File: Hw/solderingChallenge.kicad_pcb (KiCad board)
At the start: 2 copper layers, 33.5 x 33.5 mm, 28 parts, among them J1 ISP, U1 ATtiny85-20SU

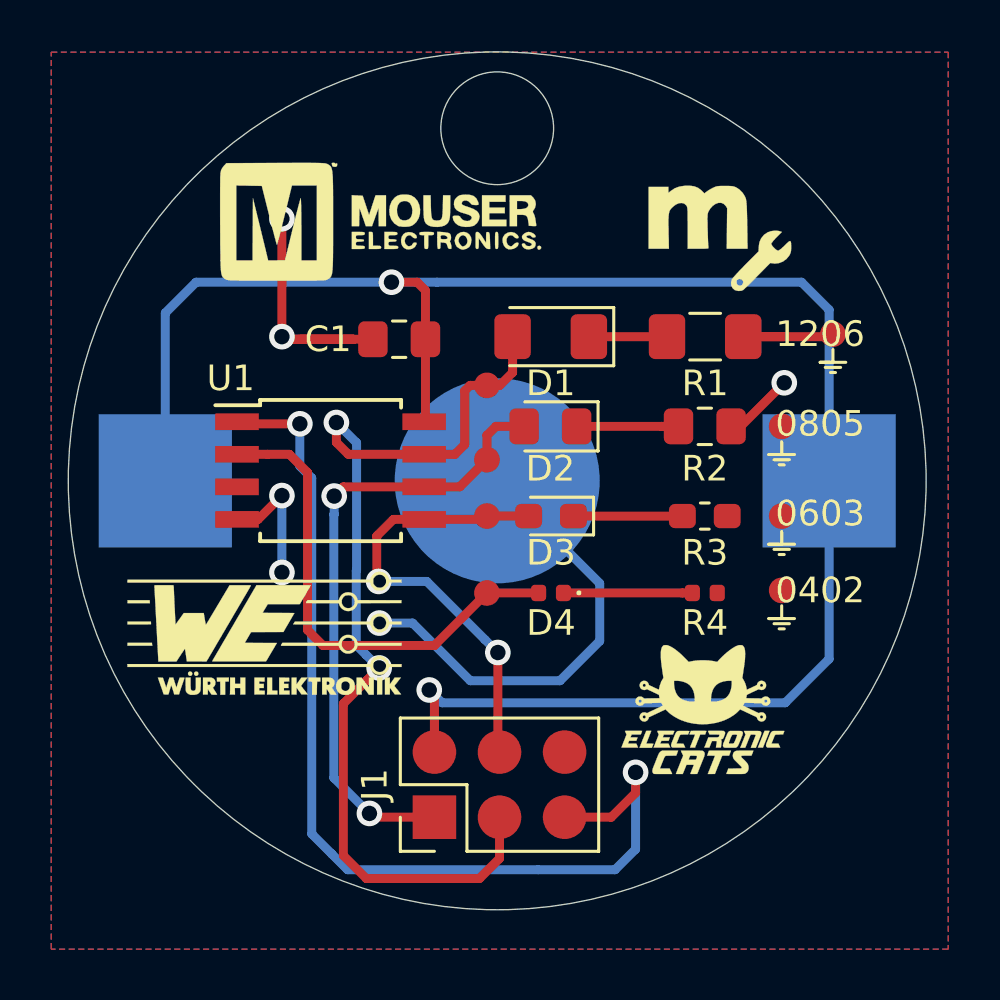
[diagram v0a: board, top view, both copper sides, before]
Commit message: feat(Hw):Added_Puya_PCB
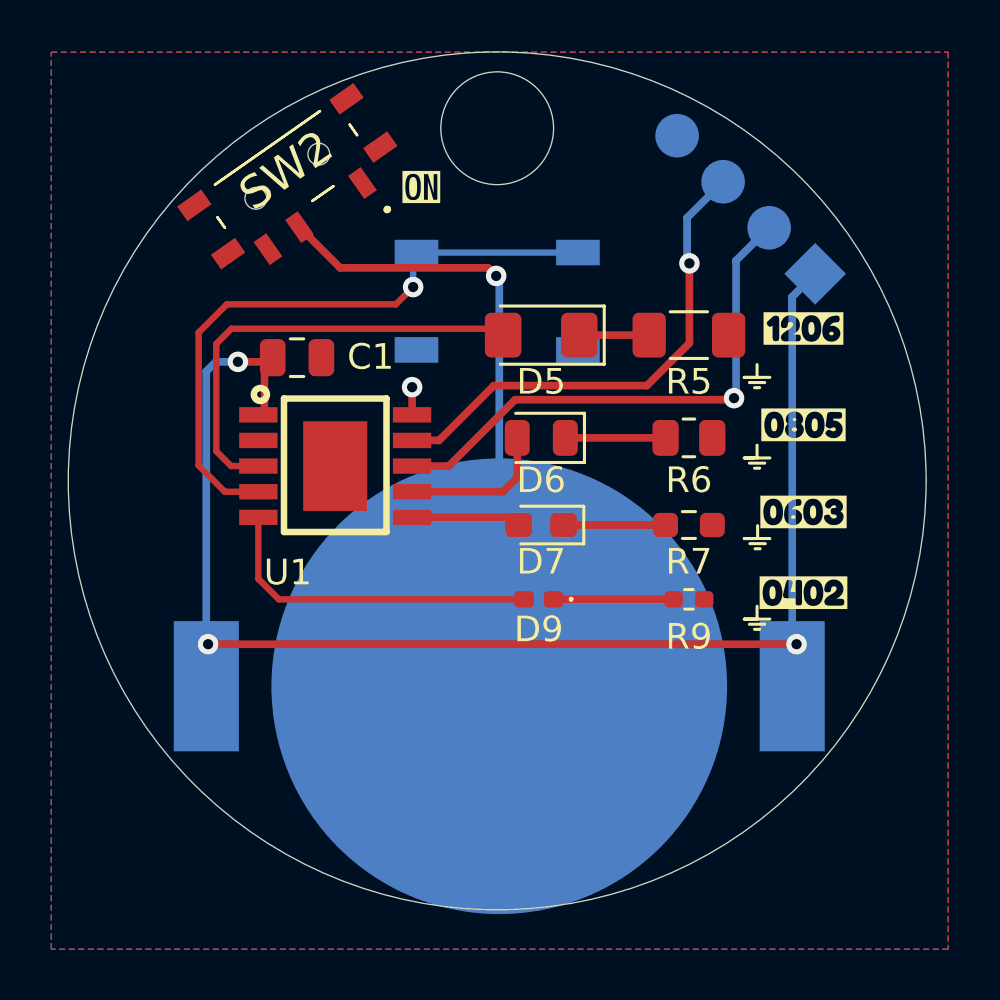
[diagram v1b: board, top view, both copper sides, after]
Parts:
- removed D1: 1206, LED_SMD:LED_1206_3216Metric_Pad1.42x1.75mm_HandSolder
- removed D2: 0805, LED_SMD:LED_0805_2012Metric_Pad1.15x1.40mm_HandSolder
- removed D3: 0603, LED_SMD:LED_0603_1608Metric_Pad1.05x0.95mm_HandSolder
- removed D4: 0402, LED_SMD:LED_0402_1005Metric
- removed the G*** at (133.6, 88.9)
- removed the G*** at (133.3, 85.2)
- removed the G*** at (150.4, 88.2)
- removed the G*** at (130.4, 73.0)
- removed the G*** at (151.4, 89.1)
- removed the G*** at (137.8, 69.1)
- removed the G*** at (142.6, 92.3)
- removed the G*** at (150.2, 69.0)
- removed J1: ISP, Connector_PinHeader_2.54mm:PinHeader_2x03_P2.54mm_Vertical
- removed R1: 1206, Resistor_SMD:R_1206_3216Metric_Pad1.42x1.75mm_HandSolder
- removed R2: 0805, Resistor_SMD:R_0805_2012Metric_Pad1.15x1.40mm_HandSolder
- removed R3: 0603, Resistor_SMD:R_0603_1608Metric_Pad1.05x0.95mm_HandSolder
- removed R4: 0402, Resistor_SMD:R_0402_1005Metric
- removed TP1: PB0, TestPoint:TestPoint_Pad_1.0x1.0mm
- removed TP10, TP6, TP7, TP8: GND, Connectors_EC:TestPoint_Pad_1.0x1.0mm
- removed TP2: PB1, Connectors_EC:TestPoint_Pad_1.0x1.0mm
- removed TP3: PB2, Connectors_EC:TestPoint_Pad_1.0x1.0mm
- removed TP4: PB3, Connectors_EC:TestPoint_Pad_1.0x1.0mm
- added D5: Green, LED_SMD:LED_1206_3216Metric_Pad1.42x1.75mm_HandSolder, F.Cu at (144.1, 73.5)
- added D6: Red, LED_SMD:LED_0805_2012Metric, F.Cu at (144.1, 77.5)
- added D7: Blue, LED_SMD:LED_0603_1608Metric_Pad1.05x0.95mm_HandSolder, F.Cu at (144.1, 81.0)
- added D9: Yellow, LED_SMD:LED_0402_1005Metric_Pad0.77x0.64mm_HandSolder, F.Cu at (144.0, 83.8)
- added G***: LOGO, Aesthetics:pcbway_13x4, F.Cu at (142.4, 88.5)
- added G***: LOGO, Aesthetics:electronic_cats_logo_4x3, F.Cu at (142.5, 92.6)
- added J2: SWD, Connector_PinHeader_2.54mm:PinHeader_1x04_P2.54mm_Vertical, B.Cu at (154.8, 71.1)
- added R5: 330R, Resistor_SMD:R_1206_3216Metric_Pad1.30x1.75mm_HandSolder, F.Cu at (149.9, 73.5)
- added R6: 330R, Resistor_SMD:R_0805_2012Metric, F.Cu at (149.9, 77.5)
- added R7: 330R, Resistor_SMD:R_0603_1608Metric_Pad0.98x0.95mm_HandSolder, F.Cu at (149.9, 81.0)
- added R9: 330R, Resistor_SMD:R_0402_1005Metric_Pad0.72x0.64mm_HandSolder, F.Cu at (149.9, 83.8)
- added SW1: SW_RST, Button_Switch_SMD:SW_SPST_TL3342, B.Cu at (142.4, 72.2)
- added SW2: On, solderingChallenge:MSK12C02, F.Cu at (134.2, 67.3)
- added kibuzzard-67914DBF: G***, kibuzzard-67914DBF, F.Cu at (154.3, 73.3)
- added kibuzzard-67914DD8: G***, kibuzzard-67914DD8, F.Cu at (154.3, 77.0)
- added kibuzzard-67914DE9: G***, kibuzzard-67914DE9, F.Cu at (154.3, 80.4)
- added kibuzzard-67914E01: G***, kibuzzard-67914E01, F.Cu at (154.3, 83.6)
- added kibuzzard-67916211: G***, kibuzzard-67916211, F.Cu at (129.1, 79.0)
- added kibuzzard-6791629E: G***, kibuzzard-6791629E, F.Cu at (129.1, 79.0)
- added kibuzzard-67916383: G***, kibuzzard-67916383, B.Cu at (153.0, 73.0)
- added kibuzzard-679163A9: G***, kibuzzard-679163A9, B.Cu at (149.4, 69.4)
- added kibuzzard-679163CD: G***, kibuzzard-679163CD, B.Cu at (151.2, 71.2)
- added kibuzzard-679168C7: G***, kibuzzard-679168C7, B.Cu at (156.0, 78.8)
- added kibuzzard-679168F3: G***, kibuzzard-679168F3, B.Cu at (147.6, 67.5)
- added kibuzzard-67916B62: G***, kibuzzard-67916B62, F.Cu at (139.4, 67.8)
- BT1: footprint Connectors_EC:79523141 -> solderingChallenge:BAT-HLD-001
- C1: footprint Capacitor_SMD:C_0805_2012Metric_Pad1.15x1.40mm_HandSolder -> Capacitor_SMD:C_0805_2012Metric
- U1: value ATtiny85-20SU -> PY32F002AA15M6TU; footprint Package_SO:SOIJ-8_5.3x5.3mm_P1.27mm -> solderingChallenge:PY32F002AA15M
- moved BT1 8.02 mm to (142.5, 87.2)
- moved C1 4.05 mm to (134.6, 74.4), turned to 0 degrees
- moved U1 0.25 mm to (136.1, 78.7)
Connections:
- BT1 pad 1: VCC -> Net-(BT1--)
- BT1 pad 2: GND -> +3.3V
- C1 pad 1: VCC -> +3.3V
- U1 pad 1: /RST -> +3.3V
- U1 pad 2: /PB3 -> /PF0
- U1 pad 3: /PB4 -> /PA5
- U1 pad 4: GND -> /NRST
- U1 pad 5: /MOSI -> /PA1
- U1 pad 6: /MISO -> /PA6
- U1 pad 7: /PB2 -> /PA7
- U1 pad 8: VCC -> /SWDIO
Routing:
- net VCC: track 74.0 -> 0.00 mm, vias 2 -> 0
- net +3.3V: track 0.00 -> 59.2 mm, vias 0 -> 3
- net GND: track 44.1 -> 1.08 mm, vias 6 -> 1
- net /RST: track 39.2 -> 0.00 mm, vias 2 -> 0
- net /PB2: track 38.4 -> 0.00 mm, vias 2 -> 0
- net /MISO: track 24.8 -> 0.00 mm, vias 2 -> 0
- net /NRST: track 0.00 -> 24.7 mm, vias 0 -> 1
- net Net-(BT1--): track 0.00 -> 24.5 mm, vias 0 -> 1
- net /SWDIO: track 0.00 -> 20.9 mm, vias 0 -> 1
- net /SWCLK: track 0.00 -> 19.3 mm, vias 0 -> 1
- net /PB3: track 19.3 -> 0.00 mm
- net /MOSI: track 17.7 -> 0.00 mm, vias 2 -> 0
- net /PA5: track 0.00 -> 17.6 mm
- net /PA1: track 0.00 -> 13.1 mm
- net /PA7: track 0.00 -> 5.87 mm
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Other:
- net class Default removed
- net class vcc removed
- board text removed: "0402"
- board text removed: "0603"
- board text removed: "0805"
- board text removed: "1206"
- board text removed: "Soldering Challenge"
- board text removed: "V1.0"
